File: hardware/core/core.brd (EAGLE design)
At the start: 141.9 x 142.2 mm, 340 parts, among them IC1 MAX481CSA, IC10 MAX481CSA, IC11 MAX481CSA, IC12 MAX481CSA, IC13 MAX481CSA, IC14 MAX481CSA, IC15 MAX481CSA, IC16 MAX481CSA, IC17 MAX481CSA, IC18 MAX481CSA, IC19 MAX481CSA, IC2 LD117AS12TR, IC20 MAX481CSA, IC21 MAX481CSA, IC22 LD117AS12TR, IC3 MAX481CSA, IC4 MAX481CSA, IC5 MAX481CSA, IC6 MAX481CSA, IC7 MAX481CSA, IC8 MAX481CSA, IC9 MAX481CSA

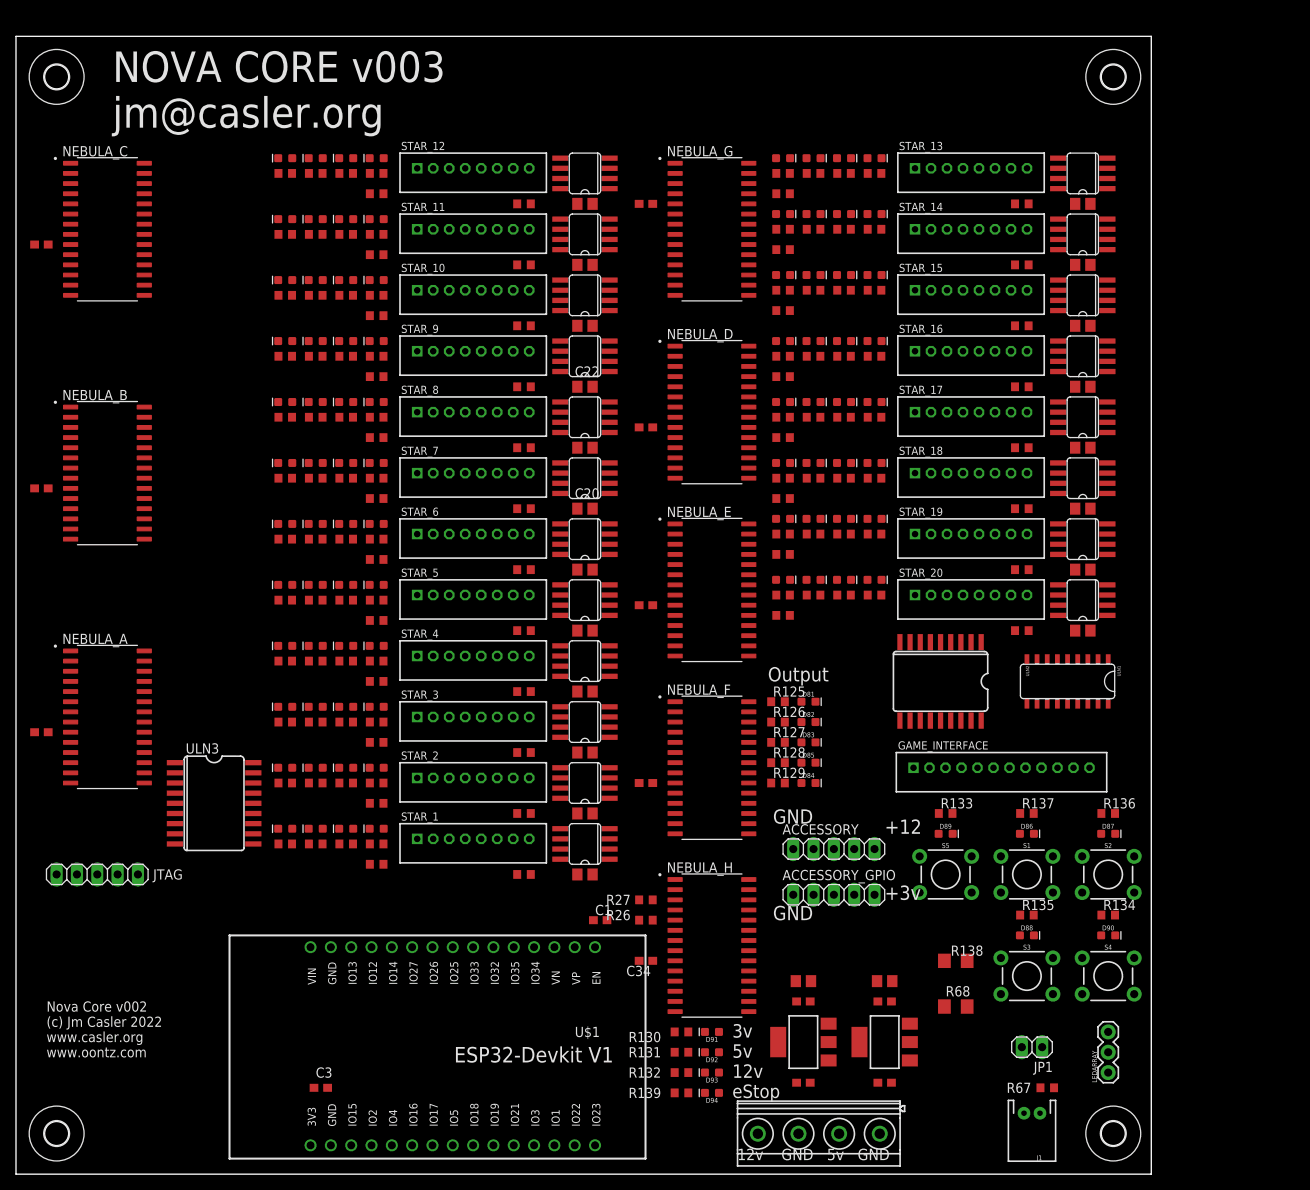
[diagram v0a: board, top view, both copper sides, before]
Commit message: More Progress
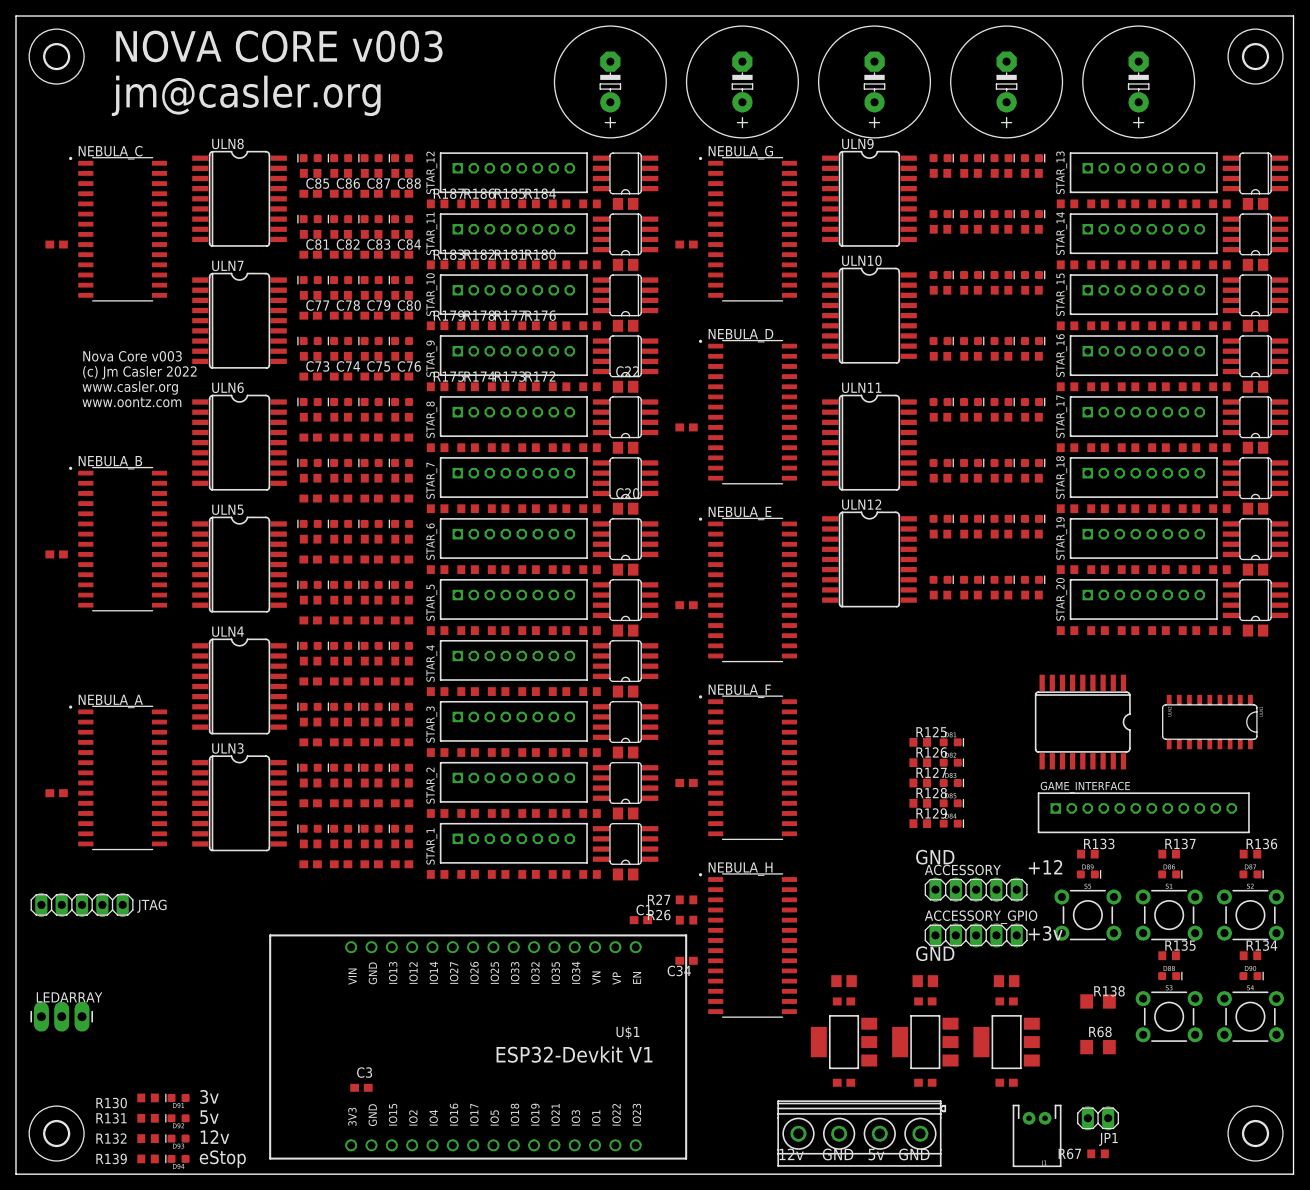
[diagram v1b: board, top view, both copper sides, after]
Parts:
- added C37, C38, C39, C40, C41, C42, C43, C44, C45, C46, C47, C48, C49, C50, C51, C52, C53, C54, C55, C56, C57, C58, C59, C60, C61, C62, C63, C64, C65, C66, C67, C68, C73, C74, C75, C76, C77, C78, C79, C80, C81, C82, C83, C84, C85, C86, C87, C88: 1nf, rcl:C0603
- added C69, C70, C71, C72, C89: 2200uf, rcl:E5-13
- added C90: 1uf, rcl:C0805
- added C91, C92: 10uf, rcl:C0603
- added IC23: LD117AS12TR, v-reg:SOT223
- added R140, R141, R142, R143, R144, R145, R146, R147, R148, R149, R150, R151, R152, R153, R154, R155, R156, R157, R158, R159, R160, R161, R162, R163, R164, R165, R166, R167, R168, R169, R170, R171, R172, R173, R174, R175, R176, R177, R178, R179, R180, R181, R182, R183, R184, R185, R186, R187, R188, R189, R190, R191, R192, R193, R194, R195, R196, R197, R198, R199, R200, R201, R202, R203, R204, R205, R206, R207, R208, R209, R210, R211, R212, R213, R214, R215, R216, R217, R218, R219: 68, rcl:R0603
- added ULN10, ULN11, ULN12, ULN4, ULN5, ULN6, ULN7, ULN8, ULN9: (no value), SparkFun-IC-Special-Function:SO18L
- LEDARRAY: device SparkFun-Connectors:1X03 -> SparkFun-Connectors:1X03_LONGPADS
- moved LEDARRAY 128.5 mm to (8.26, 19.7), turned to 180 degrees
- moved D91 67.2 mm to (20.3, 9.53)
- moved D92 67.2 mm to (20.3, 6.99)
- moved D93 67.2 mm to (20.3, 4.45)
- moved D94 67.2 mm to (20.3, 1.91)
- moved R130 67.2 mm to (16.5, 9.53)
- moved R131 67.2 mm to (16.5, 6.99)
- moved R132 67.2 mm to (16.5, 4.45)
- moved R139 67.2 mm to (16.5, 1.91)
- moved R105 50.8 mm to (146.7, 75.6)
- moved R106 50.8 mm to (146.7, 67.9)
- moved R84 50.8 mm to (146.7, 113.7)
- moved R85 50.8 mm to (146.7, 106.0)
- moved R103 50.8 mm to (146.7, 90.8)
- moved R104 50.8 mm to (146.7, 83.2)
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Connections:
- new net N$168: R143.2, STAR_1.2
- new net N$169: R142.2, STAR_1.3
- new net N$170: R141.2, STAR_1.4
- new net N$171: R140.2, STAR_1.5
- new net N$172: R147.2, STAR_2.2
- new net N$173: R146.2, STAR_2.3
- new net N$174: R145.2, STAR_2.4
- new net N$175: R144.2, STAR_2.5
- new net N$176: R151.2, STAR_3.2
- new net N$177: R150.2, STAR_3.3
- new net N$178: R149.2, STAR_3.4
- new net N$179: R148.2, STAR_3.5
- new net N$180: R155.2, STAR_4.2
- new net N$181: R154.2, STAR_4.3
- new net N$182: R153.2, STAR_4.4
- new net N$183: R152.2, STAR_4.5
- new net N$184: C45.1, R11.1, R151.1, ULN4.11
- new net N$185: C46.1, R12.1, R150.1, ULN4.12
- new net N$186: C47.1, R13.1, R149.1, ULN4.13
- new net N$187: C48.1, R14.1, R148.1, ULN4.14
- new net N$188: C52.1, R152.1, R18.1, ULN4.18
- new net N$189: C51.1, R153.1, R17.1, ULN4.17
- new net N$190: C50.1, R154.1, R16.1, ULN4.16
- new net N$191: C49.1, R15.1, R155.1, ULN4.15
- new net N$192: C53.1, R159.1, R19.1, ULN5.11
- new net N$193: C56.1, R156.1, R22.1, ULN5.14
- new net N$194: C55.1, R157.1, R21.1, ULN5.13
- new net N$195: C54.1, R158.1, R20.1, ULN5.12
- new net N$196: C60.1, R160.1, R28.1, ULN5.18
- new net N$197: C59.1, R161.1, R25.1, ULN5.17
- new net N$198: C58.1, R162.1, R24.1, ULN5.16
- new net N$199: C57.1, R163.1, R23.1, ULN5.15
- new net N$200: R159.2, STAR_5.2
- new net N$201: R158.2, STAR_5.3
- new net N$202: R157.2, STAR_5.4
- new net N$203: R156.2, STAR_5.5
- new net N$204: R163.2, STAR_6.2
- new net N$205: R162.2, STAR_6.3
- new net N$206: R161.2, STAR_6.4
- new net N$207: R160.2, STAR_6.5
- new net N$208: R167.2, STAR_7.2
- new net N$209: R166.2, STAR_7.3
- new net N$210: R165.2, STAR_7.4
- new net N$211: R164.2, STAR_7.5
- new net N$212: R171.2, STAR_8.2
- new net N$213: R170.2, STAR_8.3
- new net N$214: R169.2, STAR_8.4
- new net N$215: R168.2, STAR_8.5
- new net N$216: C61.1, R167.1, R29.1, ULN6.11
- new net N$217: C62.1, R166.1, R30.1, ULN6.12
- new net N$218: C63.1, R165.1, R31.1, ULN6.13
- new net N$219: C64.1, R164.1, R32.1, ULN6.14
- new net N$220: C68.1, R168.1, R36.1, ULN6.18
- new net N$221: C67.1, R169.1, R35.1, ULN6.17
- new net N$222: C66.1, R170.1, R34.1, ULN6.16
- new net N$223: C65.1, R171.1, R33.1, ULN6.15
- new net N$224: R175.2, STAR_9.2
- new net N$225: R179.2, STAR_10.2
- new net N$226: R178.2, STAR_10.3
- new net N$227: R174.2, STAR_9.3
- new net N$228: R173.2, STAR_9.4
- new net N$229: R172.2, STAR_9.5
- new net N$230: R177.2, STAR_10.4
- new net N$231: R176.2, STAR_10.5
- new net N$232: R183.2, STAR_11.2
- new net N$233: R182.2, STAR_11.3
- new net N$234: R181.2, STAR_11.4
- new net N$235: R180.2, STAR_11.5
- new net N$236: R187.2, STAR_12.2
- new net N$237: R186.2, STAR_12.3
- new net N$238: R185.2, STAR_12.4
- new net N$239: R184.2, STAR_12.5
- new net N$240: C73.1, R175.1, R37.1, ULN7.11
- new net N$241: C74.1, R174.1, R38.1, ULN7.12
- new net N$242: C75.1, R173.1, R39.1, ULN7.13
- new net N$243: C76.1, R172.1, R40.1, ULN7.14
- new net N$244: R191.2, STAR_13.2
- new net N$245: C79.1, R177.1, R43.1, ULN7.17
- new net N$246: C78.1, R178.1, R42.1, ULN7.16
- new net N$247: C77.1, R179.1, R41.1, ULN7.15
- new net N$248: C81.1, R183.1, R45.1, ULN8.11
- new net N$249: C82.1, R182.1, R46.1, ULN8.12
- new net N$250: C83.1, R181.1, R47.1, ULN8.13
- new net N$251: C84.1, R180.1, R48.1, ULN8.14
- new net N$252: C80.1, R176.1, R44.1, ULN7.18
- new net N$253: C87.1, R185.1, R51.1, ULN8.17
- new net N$254: C86.1, R186.1, R50.1, ULN8.16
- new net N$255: C85.1, R187.1, R49.1, ULN8.15
- new net N$256: R190.2, STAR_13.3
- new net N$257: R189.2, STAR_13.4
- new net N$258: R188.2, STAR_13.5
- new net N$259: R196.2, STAR_14.2
- new net N$260: C88.1, R184.1, R52.1, ULN8.18
- new net N$261: R195.2, STAR_14.3
- new net N$262: R194.2, STAR_14.4
- new net N$263: R193.2, STAR_14.5
- new net N$264: R199.2, STAR_15.2
- new net N$265: R198.2, STAR_15.3
- new net N$266: R192.2, STAR_15.5
- new net N$267: R197.2, STAR_15.4
- new net N$268: R203.2, STAR_16.2
- new net N$269: R202.2, STAR_16.3
- new net N$270: R201.2, STAR_16.4
- new net N$271: R200.2, STAR_16.5
- new net N$272: R216.2, STAR_20.5
- new net N$273: R217.2, STAR_20.4
- new net N$274: R218.2, STAR_20.3
- new net N$275: R219.2, STAR_20.2
- new net N$276: R212.2, STAR_19.5
- new net N$277: R213.2, STAR_19.4
- new net N$278: R214.2, STAR_19.3
- new net N$279: R215.2, STAR_19.2
- new net N$280: R208.2, STAR_18.5
- new net N$281: R209.2, STAR_18.4
- new net N$282: R210.2, STAR_18.3
- new net N$283: R211.2, STAR_18.2
- new net N$284: R204.2, STAR_17.5
- new net N$285: R205.2, STAR_17.4
- new net N$286: R206.2, STAR_17.3
- new net N$287: R207.2, STAR_17.2
- net +12V: now also C89.+, C90.1, C92.1, IC23.3, ULN4.10, ULN5.10, ULN6.10, ULN7.10, ULN8.10
- net +3V3: now also C70.+, C72.+
- net +5V: now also C69.+, C71.+, C91.1, D10.A, D11.A, D12.A, D13.A, D14.A, D15.A, D16.A, D17.A, D18.A, D19.A, D20.A, D21.A, D22.A, D23.A, D24.A, D25.A, D26.A, D27.A, D28.A, D29.A, D30.A, D31.A, D32.A, D33.A, D34.A, D35.A, D36.A, D37.A, D38.A, D39.A, D40.A, D41.A, D42.A, D43.A, D44.A, D45.A, D46.A, D47.A, D48.A, D49.A, IC23.4
- net A10: now also ULN4.6; no longer D12.A, STAR_3.4
- net A11: now also ULN4.5; no longer D13.A, STAR_3.5
- net A12: now also ULN4.4; no longer D14.A, STAR_4.2
- net A13: now also ULN4.3; no longer D15.A, STAR_4.3
- net A14: now also ULN4.2; no longer D16.A, STAR_4.4
- net A15: now also ULN4.1; no longer D17.A, STAR_4.5
- net A8: now also ULN4.8; no longer D10.A, STAR_3.2
- net A9: now also ULN4.7; no longer D11.A, STAR_3.3
- net B0: now also ULN5.8; no longer D18.A, STAR_5.2
- net B1: now also ULN5.7; no longer D19.A, STAR_5.3
- net B10: now also ULN6.6; no longer D28.A, STAR_7.4
- net B11: now also ULN6.5; no longer D29.A, STAR_7.5
- net B12: now also ULN6.4; no longer D30.A, STAR_8.2
- net B13: now also ULN6.3; no longer D31.A, STAR_8.3
- net B14: now also ULN6.2; no longer D32.A, STAR_8.4
- net B15: now also ULN6.1; no longer D33.A, STAR_8.5
- net B2: now also ULN5.6; no longer D20.A, STAR_5.4
- net B3: now also ULN5.5; no longer D21.A, STAR_5.5
- net B4: now also ULN5.4; no longer D22.A, STAR_6.2
- net B5: now also ULN5.3; no longer D23.A, STAR_6.3
- net B6: now also ULN5.2; no longer D24.A, STAR_6.4
- net B7: now also ULN5.1; no longer D25.A, STAR_6.5
- net B8: now also ULN6.8; no longer D26.A, STAR_7.2
- net B9: now also ULN6.7; no longer D27.A, STAR_7.3
- net C0: now also ULN7.8; no longer D34.A, STAR_9.2
- net C1: now also ULN7.7; no longer D35.A, STAR_9.3
- net C10: now also ULN8.6; no longer D44.A, STAR_11.4
- net C11: now also ULN8.5; no longer D45.A, STAR_11.5
- net C12: now also ULN8.4; no longer D46.A, STAR_12.2
- net C13: now also ULN8.3; no longer D47.A, STAR_12.3
- net C14: now also ULN8.2; no longer D48.A, STAR_12.4
- net C15: now also ULN8.1; no longer D49.A, STAR_12.5
- net C2: now also ULN7.6; no longer D36.A, STAR_9.4
- net C3: now also ULN7.5; no longer D37.A, STAR_9.5
- net C4: now also ULN7.4; no longer D38.A, STAR_10.2
- net C5: now also ULN7.3; no longer D39.A, STAR_10.3
- net C6: now also ULN7.2; no longer D40.A, STAR_10.4
- net C7: now also ULN7.1; no longer D41.A, STAR_10.5
- net C8: now also ULN8.8; no longer D42.A, STAR_11.2
- net C9: now also ULN8.7; no longer D43.A, STAR_11.3
- net D0: no longer D1.A, STAR_13.2
- net D1: no longer D50.A, STAR_13.3
- net D10: no longer D59.A, STAR_15.4
- net D11: no longer D60.A, STAR_15.5
- net D12: no longer D61.A, STAR_16.2
- net D13: no longer D62.A, STAR_16.3
- net D14: no longer D63.A, STAR_16.4
- net D15: no longer D64.A, STAR_16.5
- net D2: no longer D51.A, STAR_13.4
- net D3: no longer D52.A, STAR_13.5
- net D4: no longer D53.A, STAR_14.2
- net D5: no longer D54.A, STAR_14.3
- net D6: no longer D55.A, STAR_14.4
- net D7: no longer D56.A, STAR_14.5
- net D8: no longer D57.A, STAR_15.2
- net D9: no longer D58.A, STAR_15.3
- net E0: no longer D65.A, STAR_17.2
- net E1: no longer D66.A, STAR_17.3
- net E10: no longer D75.A, STAR_19.4
- net E11: no longer D76.A, STAR_19.5
- net E12: no longer D77.A, STAR_20.2
- net E13: no longer D78.A, STAR_20.3
- net E14: no longer D79.A, STAR_20.4
- net E15: no longer D80.A, STAR_20.5
- net E2: no longer D67.A, STAR_17.4
- net E3: no longer D68.A, STAR_17.5
- net E4: no longer D69.A, STAR_18.2
- net E5: no longer D70.A, STAR_18.3
- net E6: no longer D71.A, STAR_18.4
- net E7: no longer D72.A, STAR_18.5
- net E8: no longer D73.A, STAR_19.2
- net E9: no longer D74.A, STAR_19.3
- net GND: now also C37.2, C38.2, C39.2, C40.2, C41.2, C42.2, C43.2, C44.2, C45.2, C46.2, C47.2, C48.2, C49.2, C50.2, C51.2, C52.2, C53.2, C54.2, C55.2, C56.2, C57.2, C58.2, C59.2, C60.2, C61.2, C62.2, C63.2, C64.2, C65.2, C66.2, C67.2, C68.2, C69.-, C70.-, C71.-, C72.-, C73.2, C74.2, C75.2, C76.2, C77.2, C78.2, C79.2, C80.2, C81.2, C82.2, C83.2, C84.2, C85.2, C86.2, C87.2, C88.2, C89.-, C90.2, C91.2, C92.2, IC23.1, ULN4.9, ULN5.9, ULN6.9, ULN7.9, ULN8.9; no longer R11.1, R12.1, R13.1, R14.1, R15.1, R16.1, R17.1, R18.1, R19.1, R20.1, R21.1, R22.1, R23.1, R24.1, R25.1, R28.1, R29.1, R30.1, R31.1, R32.1, R33.1, R34.1, R35.1, R36.1, R37.1, R38.1, R39.1, R40.1, R41.1, R42.1, R43.1, R44.1, R45.1, R46.1, R47.1, R48.1, R49.1, R50.1, R51.1, R52.1
- net N$160: now also C37.1, R143.1; no longer STAR_1.2
- net N$161: now also C38.1, R142.1; no longer STAR_1.3
- net N$162: now also C39.1, R141.1; no longer STAR_1.4
- net N$163: now also C40.1, R140.1; no longer STAR_1.5
- net N$164: now also C44.1, R144.1; no longer STAR_2.5
- net N$165: now also C43.1, R145.1; no longer STAR_2.4
- net N$166: now also C42.1, R146.1; no longer STAR_2.3
- net N$167: now also C41.1, R147.1; no longer STAR_2.2
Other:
- board size 141.9 x 142.2 mm -> 159.7 x 144.8 mm
- board text added: "+5 DATA GND"
- board text added: "Nova Core v003 (c) Jm Casler 2022 www.casler.org www.oontz.com"
- board text removed: "Nova Core v002 (c) Jm Casler 2022 www.casler.org www.oontz.com"
- board text removed: "Output"
